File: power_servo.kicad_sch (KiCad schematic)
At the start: 120 parts, among them U10 TPS563201, U3 TPS563201, U4 TPS563201, U5 TPS563201, U6 TPS563201, U7 TPS563201, U8 TPS563201, U9 TPS563201

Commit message: update
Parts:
- D10, D11, D12, D13, D14, D7, D8, D9: footprint LED_SMD:LED_0603_1608Metric -> LED_SMD:LED_0805_2012Metric
- R76, R77, R78, R79, R80, R81, R82, R83: footprint Resistor_SMD:R_0603_1608Metric -> Resistor_SMD:R_0805_2012Metric
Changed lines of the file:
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@@
 			)
 		)
-		(property "Footprint" "Resistor_SMD:R_0603_1608Metric"
+		(property "Footprint" "Resistor_SMD:R_0805_2012Metric"
 			(at 215.9 134.62 0)
 			(effects
@@
 			)
 		)
-		(property "Footprint" "LED_SMD:LED_0603_1608Metric"
+		(property "Footprint" "LED_SMD:LED_0805_2012Metric"
 			(at 227.33 83.82 0)
 			(effects
@@
 			)
 		)
-		(property "Footprint" "Resistor_SMD:R_0603_1608Metric"
+		(property "Footprint" "Resistor_SMD:R_0805_2012Metric"
 			(at 86.36 184.15 0)
 			(effects
@@
 			)
 		)
-		(property "Footprint" "LED_SMD:LED_0603_1608Metric"
+		(property "Footprint" "LED_SMD:LED_0805_2012Metric"
 			(at 95.25 184.15 0)
 			(effects
@@
 			)
 		)
-		(property "Footprint" "Resistor_SMD:R_0603_1608Metric"
+		(property "Footprint" "Resistor_SMD:R_0805_2012Metric"
 			(at 214.63 182.88 0)
 			(effects
@@
 			)
 		)
-		(property "Footprint" "LED_SMD:LED_0603_1608Metric"
+		(property "Footprint" "LED_SMD:LED_0805_2012Metric"
 			(at 93.98 229.87 0)
 			(effects
@@
 			)
 		)
-		(property "Footprint" "Resistor_SMD:R_0603_1608Metric"
+		(property "Footprint" "Resistor_SMD:R_0805_2012Metric"
 			(at 215.9 231.14 0)
 			(effects
@@
 			)
 		)
-		(property "Footprint" "Resistor_SMD:R_0603_1608Metric"
+		(property "Footprint" "Resistor_SMD:R_0805_2012Metric"
 			(at 92.71 82.55 0)
 			(effects
@@
 			)
 		)
-		(property "Footprint" "LED_SMD:LED_0603_1608Metric"
+		(property "Footprint" "LED_SMD:LED_0805_2012Metric"
 			(at 223.52 182.88 0)
 			(effects
@@
 			)
 		)
-		(property "Footprint" "LED_SMD:LED_0603_1608Metric"
+		(property "Footprint" "LED_SMD:LED_0805_2012Metric"
 			(at 224.79 231.14 0)
 			(effects
@@
 			)
 		)
-		(property "Footprint" "LED_SMD:LED_0603_1608Metric"
+		(property "Footprint" "LED_SMD:LED_0805_2012Metric"
 			(at 224.79 134.62 0)
 			(effects
@@
 			)
 		)
-		(property "Footprint" "Resistor_SMD:R_0603_1608Metric"
+		(property "Footprint" "Resistor_SMD:R_0805_2012Metric"
 			(at 85.09 229.87 0)
 			(effects
@@
 			)
 		)
-		(property "Footprint" "LED_SMD:LED_0603_1608Metric"
+		(property "Footprint" "LED_SMD:LED_0805_2012Metric"
 			(at 101.6 82.55 0)
 			(effects
@@
 			)
 		)
-		(property "Footprint" "Resistor_SMD:R_0603_1608Metric"
+		(property "Footprint" "Resistor_SMD:R_0805_2012Metric"
 			(at 218.44 83.82 0)
 			(effects
@@
 			)
 		)
-		(property "Footprint" "Resistor_SMD:R_0603_1608Metric"
+		(property "Footprint" "Resistor_SMD:R_0805_2012Metric"
 			(at 92.71 133.35 0)
 			(effects
@@
 			)
 		)
-		(property "Footprint" "LED_SMD:LED_0603_1608Metric"
+		(property "Footprint" "LED_SMD:LED_0805_2012Metric"
 			(at 101.6 133.35 0)
 			(effects

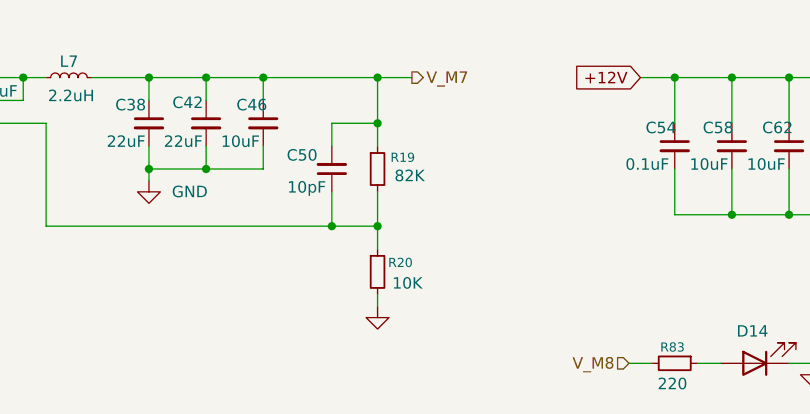
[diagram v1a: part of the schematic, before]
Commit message: update
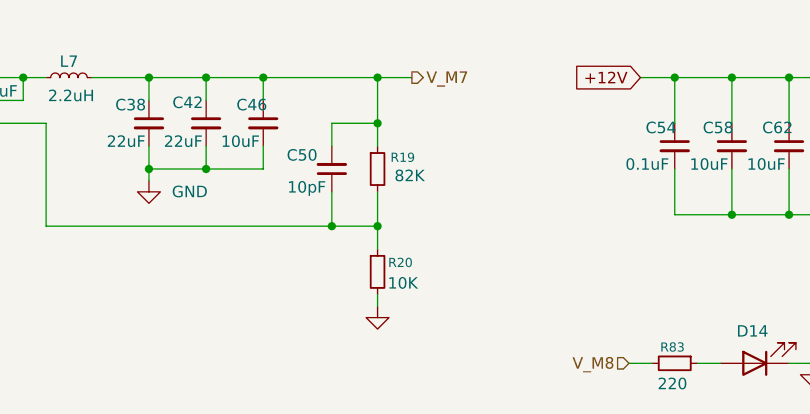
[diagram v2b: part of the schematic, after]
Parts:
- C19, C20, C21, C22, C23, C24, C25, C26, C27, C28, C29, C30, C31, C32, C33, C34, C35, C36, C37, C38, C39, C40, C41, C42, C43, C44, C45, C46, C47, C48, C49, C50, C51, C52, C53, C54, C55, C56, C57, C58, C59, C60, C61, C62, C63, C64, C65, C66, C67, C68, C69, C70, C71, C72, C73, C74, C75, C76, C77, C78, C79, C80, C81, C82: footprint Capacitor_SMD:C_0603_1608Metric -> Capacitor_SMD:C_0805_2012Metric
- R10, R11, R12, R13, R14, R15, R16, R17, R18, R19, R20, R21, R22, R23, R24, R25, R26, R27, R28, R29, R30, R31, R32, R9: footprint Resistor_SMD:R_0603_1608Metric -> Resistor_SMD:R_0805_2012Metric
